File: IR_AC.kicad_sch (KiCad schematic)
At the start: 1 part

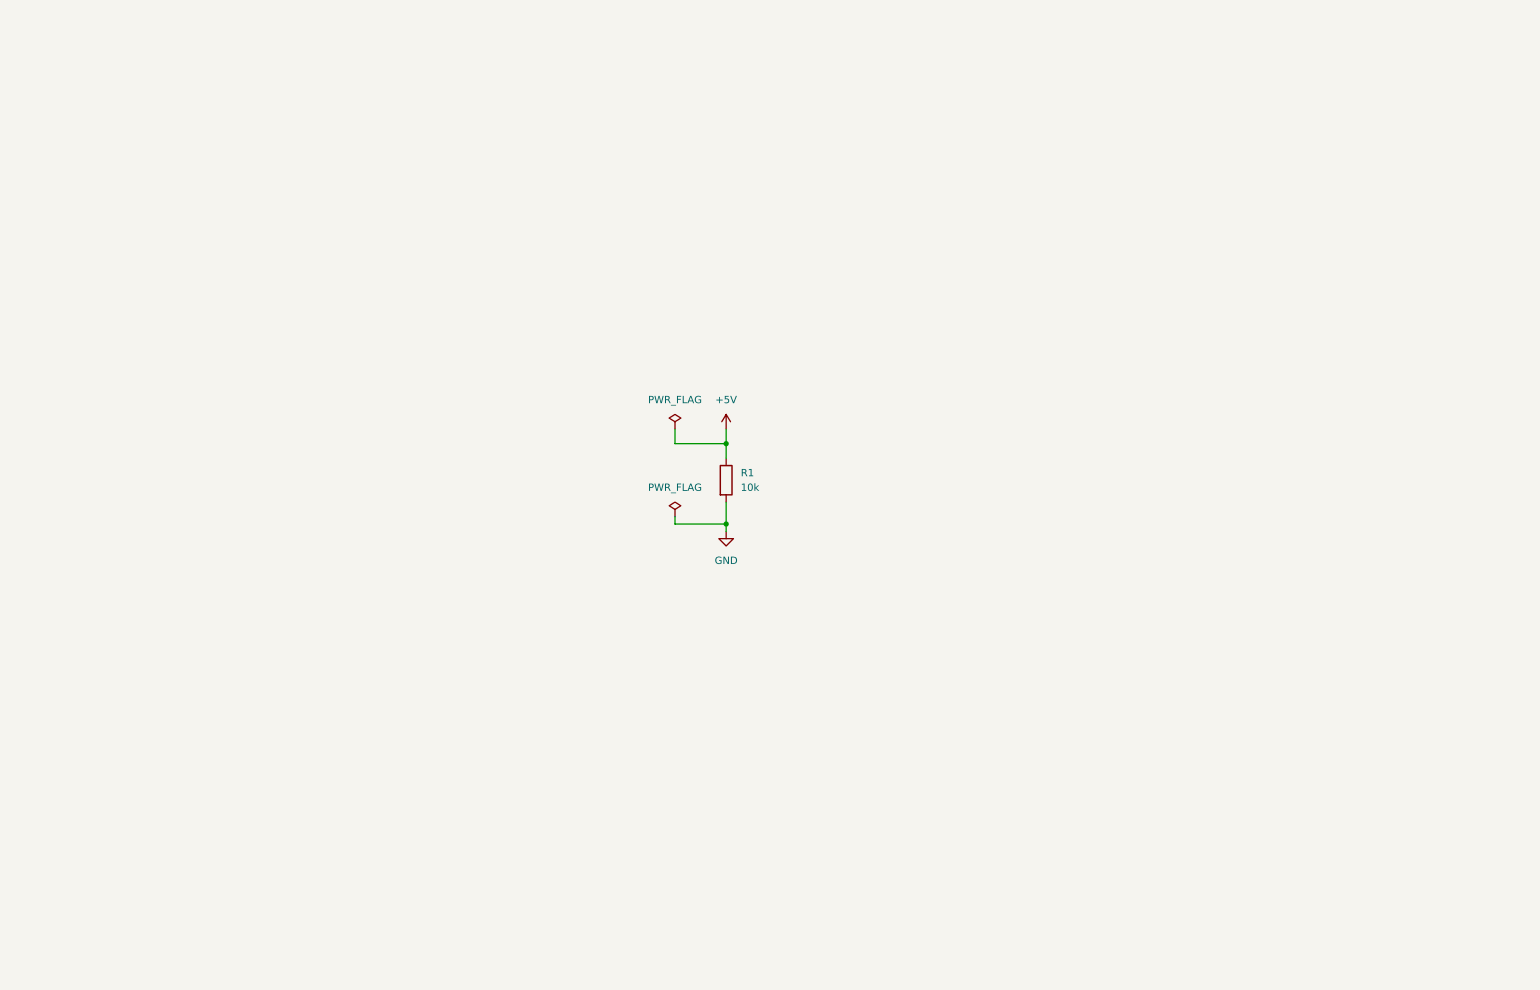
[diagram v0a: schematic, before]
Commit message: late night work on led current
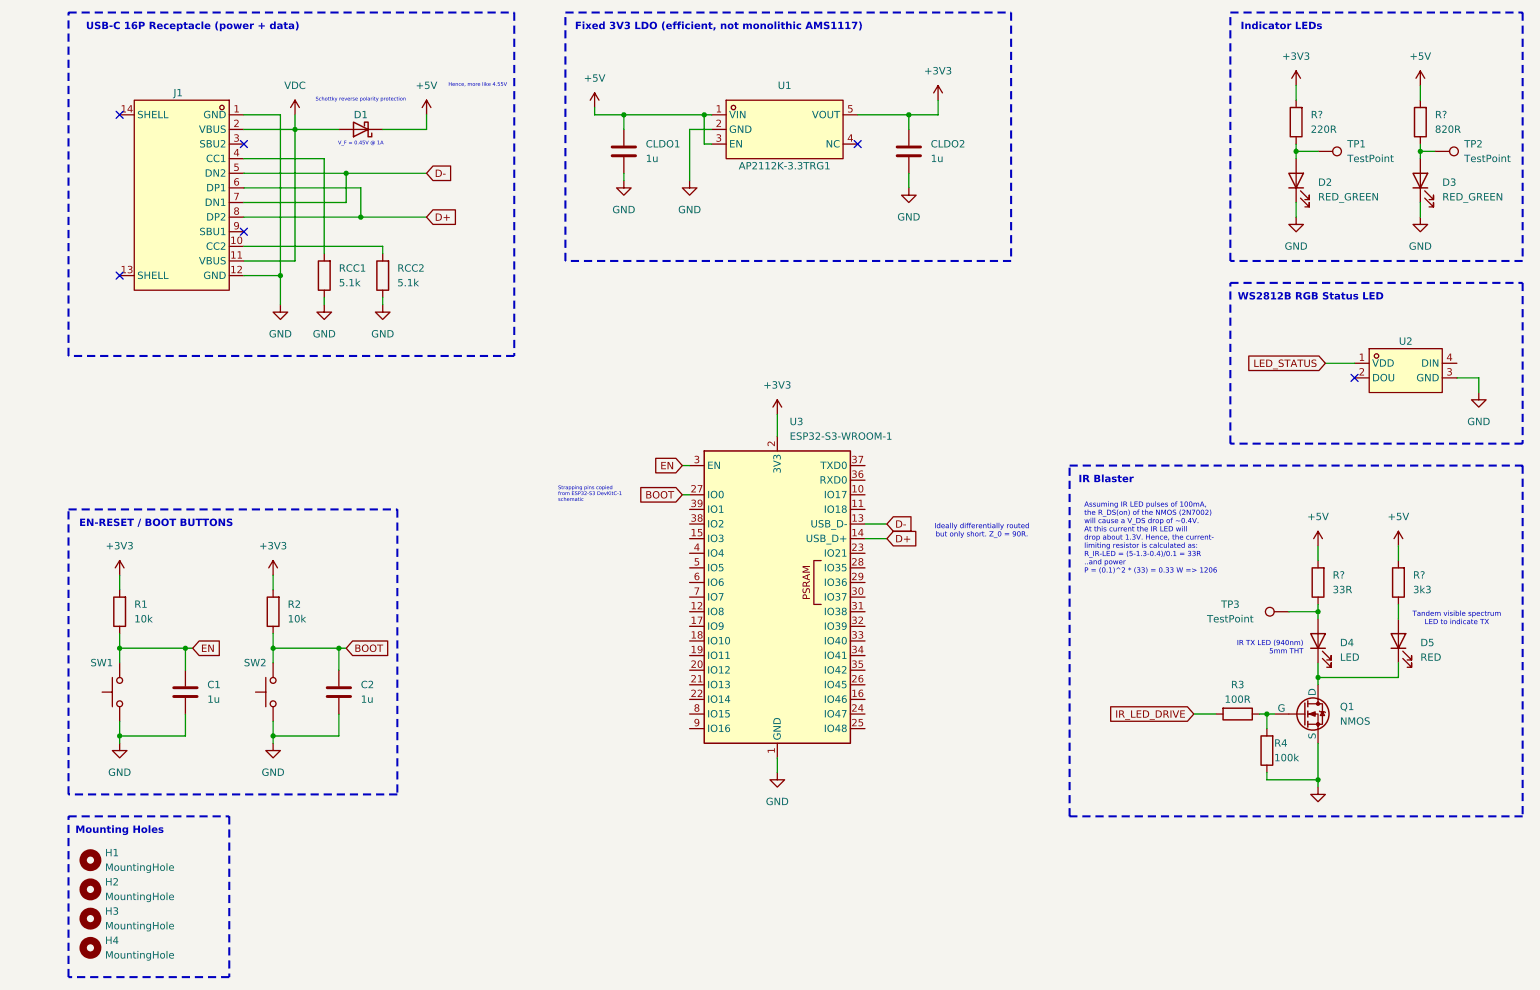
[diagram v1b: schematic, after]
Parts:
- added C1, C2: 1u, Capacitor_SMD:C_0603_1608Metric, symbol Device:C
- added CLDO1, CLDO2: 1u, Capacitor_SMD:C_0805_2012Metric, symbol Device:C
- added D1: 1N5819HW, LC_libz_foot:1N5819HW, symbol Device:D_Schottky
- added D2, D3: RED_GREEN, LED_SMD:LED_0805_2012Metric, symbol Device:LED
- added D4: LED, LC_libz_foot:IR_LED_TH_5MM, symbol Device:LED
- added D5: RED, LED_SMD:LED_0805_2012Metric, symbol Device:LED
- added H1, H2, H3, H4: MountingHole, MountingHole:MountingHole_3.2mm_M3, symbol Mechanical:MountingHole
- added J1: TYPE-C 16PIN 2MD(073), LC_libz_foot:USB-C-SMD_TYPE-C-6PIN-2MD-073, symbol LC_libz_sym:TYPE-C16PIN2MD(073)
- added Q1: NMOS, Package_TO_SOT_SMD:SOT-23, symbol Simulation_SPICE:NMOS
- added R2: 10k, Resistor_SMD:R_0603_1608Metric, symbol Device:R
- added R3: 100R, Resistor_SMD:R_0603_1608Metric, symbol Device:R
- added R4: 100k, Resistor_SMD:R_0603_1608Metric, symbol Device:R
- added R?: 3k3, Resistor_SMD:R_0603_1608Metric, symbol Device:R
- added R?: 220R, Resistor_SMD:R_0603_1608Metric, symbol Device:R
- added R?: 820R, Resistor_SMD:R_0603_1608Metric, symbol Device:R
- added R?: 33R, Resistor_SMD:R_1206_3216Metric, symbol Device:R
- added RCC1, RCC2: 5.1k, Resistor_SMD:R_0603_1608Metric, symbol Device:R
- added SW1, SW2: SW_Push, LC_libz_foot:BTN_L45_W45, symbol Switch:SW_Push
- added TP1, TP2, TP3: TestPoint, TestPoint:TestPoint_THTPad_D1.5mm_Drill0.7mm, symbol Connector:TestPoint
- added U1: AP2112K-3.3TRG1, LC_libz_foot:AP2112K-3.3, symbol LC_libz_sym:AP2112K-3.3TRG1
- added U2: WS2812B_5050, LC_libz_foot:WS2812B_5050, symbol LC_libz_sym:WS2812B_5050
- added U3: ESP32-S3-WROOM-1, RF_Module:ESP32-S3-WROOM-1, symbol RF_Module:ESP32-S3-WROOM-1
- R1: LCSC C2930027 -> C25804
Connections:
- net +5V: now also CLDO1.1, D1.1 (K), R?.2, R?.2, R?.2, U1.1 (VIN), U1.3 (EN); no longer R1.1
- net GND: now also C1.2, C2.2, CLDO1.2, CLDO2.2, D2.1 (K), D3.1 (K), J1.1 (GND), J1.12 (GND), Q1.3 (S), R4.1, RCC1.1, RCC2.1, SW1.1, SW2.1, U1.2 (GND), U2.3 (GND), U3.1 (GND), U3.40 (GND), U3.41 (GND); no longer R1.2
- new net: D3.2 (A), R?.1, TP2.1
- new net: D5.2 (A), R?.1
- new net: D2.2 (A), R?.1, TP1.1
- new net: J1.10 (CC2), RCC2.2
- new net: J1.4 (CC1), RCC1.2
- new net: D4.1 (K), D5.1 (K), Q1.1 (D)
- new net: Q1.2 (G), R3.1, R4.2
- new net: D4.2 (A), R?.1, TP3.1
- new net +3V3: CLDO2.1, R1.2, R2.2, R?.2, U1.5 (VOUT), U3.2 (3V3)
- new net BOOT: C2.1, R2.1, SW2.2, U3.27 (IO0)
- new net D+: J1.6 (DP1), J1.8 (DP2), U3.14 (USB_D+)
- new net D-: J1.5 (DN2), J1.7 (DN1), U3.13 (USB_D-)
- new net EN: C1.1, R1.1, SW1.2, U3.3 (EN)
- new net IR_LED_DRIVE: R3.2
- new net LED_STATUS: U2.1 (VDD)
- new net VDC: D1.2 (A), J1.11 (VBUS), J1.2 (VBUS)
- no-connect marks 0 -> 6
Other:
- note added: "Assuming IR LED pulses of 100mA, the R_DS(on) of the NMOS (2N7002) will cause a V_DS drop of ~0.4V. At this current the IR LED will drop about 1.3V. Hence, the current- limiting resistor is calculated as: R_IR-LED = (5-1.3-0.4)/0.1 = 33R ..and power P = (0.1)^2 * (33) = 0.33 W => 1206"
- note added: "EN-RESET / BOOT BUTTONS"
- note added: "Fixed 3V3 LDO (efficient, not monolithic AMS1117)"
- note added: "Hence, more like 4.55V"
- note added: "IR Blaster"
- note added: "IR TX LED (940nm) 5mm THT"
- note added: "Ideally differentially routed but only short. Z_0 = 90R."
- note added: "Indicator LEDs"
- note added: "Mounting Holes"
- note added: "Schottky reverse polarity protection"
- note added: "Strapping pins copied from ESP32-S3 DevKitC-1 schematic"
- note added: "Tandem visible spectrum LED to indicate TX"
- note added: "USB-C 16P Receptacle (power + data)"
- note added: "V_F = 0.45V @ 1A"
- note added: "WS2812B RGB Status LED"

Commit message: Finished schematic
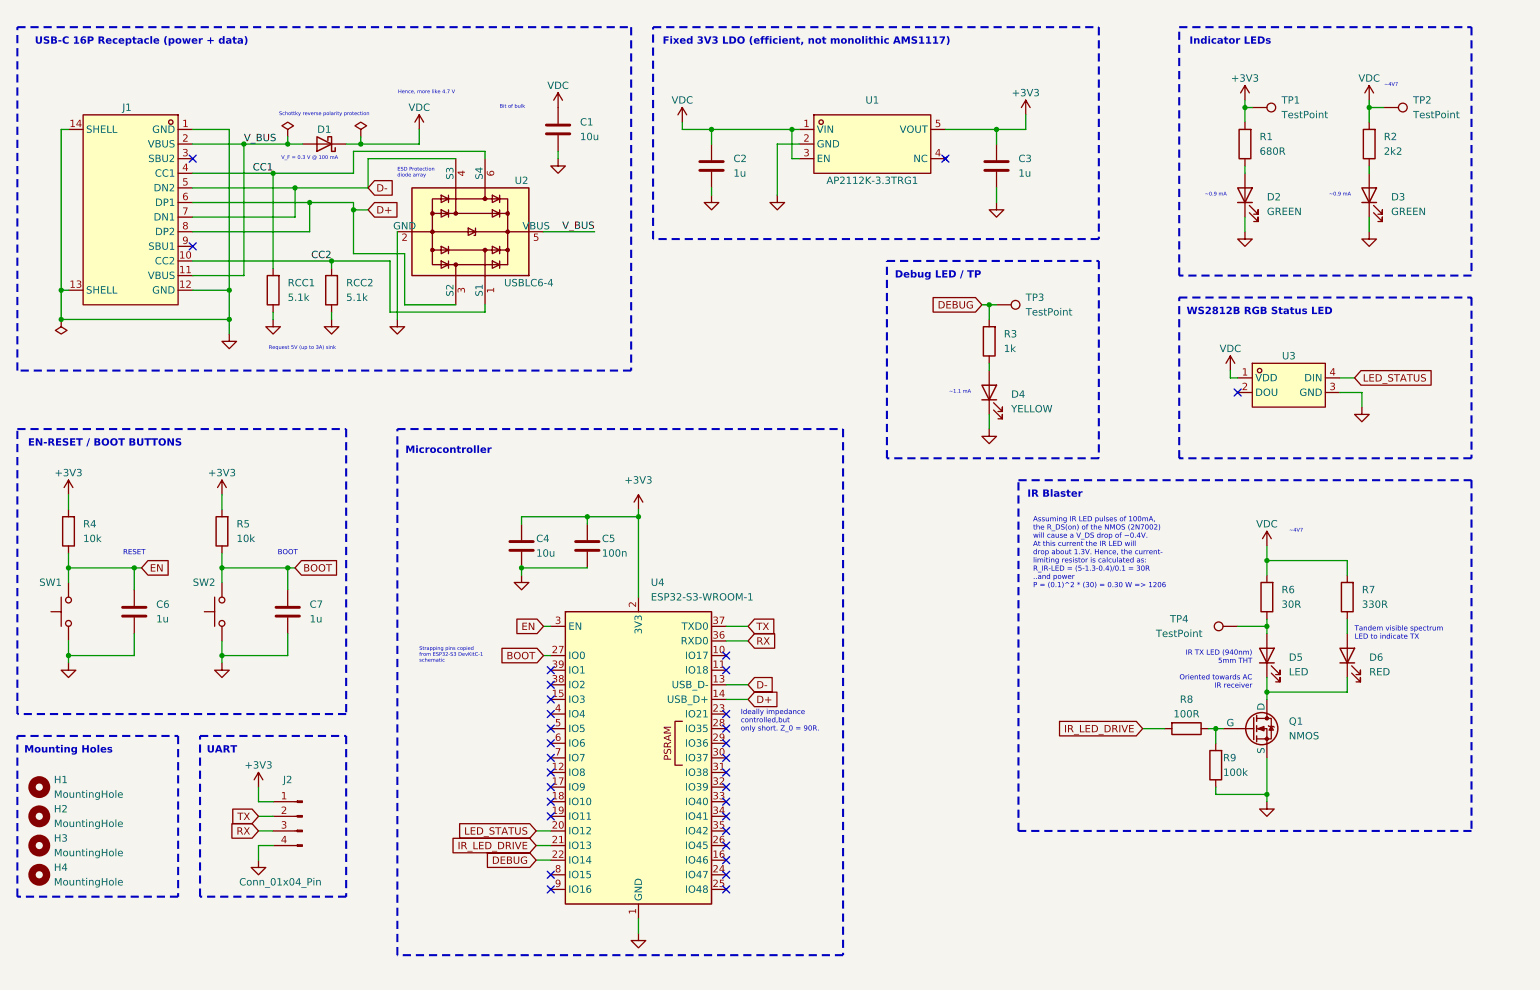
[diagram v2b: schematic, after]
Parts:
- added C1, C4: 10u, Capacitor_SMD:C_0805_2012Metric, symbol Device:C
- added C5: 100n, Capacitor_SMD:C_0402_1005Metric, symbol Device:C
- added D4: YELLOW, LED_SMD:LED_0805_2012Metric, symbol Device:LED
- added J2: Conn_01x04_Pin, libs:HDR-TH_4P-P2.54-V-M, symbol Connector:Conn_01x04_Pin
- added R3: 1k, Resistor_SMD:R_0603_1608Metric, symbol Device:R
- added TP3: TestPoint, TestPoint:TestPoint_THTPad_D1.5mm_Drill0.7mm, symbol Connector:TestPoint
- added U2: USBLC6-4, Package_TO_SOT_SMD:SOT-23-6, symbol Power_Protection:SRV05-4
- D2, D3: value RED_GREEN -> GREEN
- D6: renamed from D5; LCSC NULL -> C84256
- H1, H2, H3, H4: footprint MountingHole:MountingHole_3.2mm_M3 -> MountingHole:MountingHole_2.2mm_M2
- J1: footprint LC_libz_foot:USB-C-SMD_TYPE-C-6PIN-2MD-073 -> libs:USB-C-SMD_TYPE-C-6PIN-2MD-073
- R1: renamed from R?; value 220R -> 680R; LCSC C22962 -> C23228
- R2: renamed from R?; value 820R -> 2k2; LCSC C23253 -> C4190
- R6: renamed from R?; value 33R -> 30R; LCSC C18005 -> C25373
- R7: renamed from R?; value 3k3 -> 330R; LCSC C22978 -> C23138
- SW1, SW2: footprint LC_libz_foot:BTN_L45_W45 -> (none); LCSC C455243 -> C720477
- U1: footprint LC_libz_foot:AP2112K-3.3 -> libs:SOT-25-5_L2.9-W1.6-P0.95-LS2.8-BL
- renumbered CLDO1 to C2, CLDO2 to C3, C1 to C6, C2 to C7, D4 to D5, R1 to R4, R2 to R5, R3 to R8, R4 to R9, TP3 to TP4, U2 to U3, U3 to U4
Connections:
- net +5V is gone; now on net VDC: C2.1, D1.1 (K), R2.2, R6.2, R7.2, U1.1 (VIN), U1.3 (EN)
- net +3V3: now also TP1.1, C4.1, C5.1, J2.1 (Pin_1)
- net D+: now also U2.3 (S2)
- net D-: now also U2.4 (S3)
- net GND: now also J1.13 (SHELL), J1.14 (SHELL), C1.2, C4.2, C5.2, D4.1 (K), J2.4 (Pin_4), U2.2 (GND)
- net IR_LED_DRIVE: now also U4.21 (IO13)
- net LED_STATUS: now also U3.4 (DIN), U4.20 (IO12); no longer U3.1 (VDD)
- net VDC: now also TP2.1, U3.1 (VDD), C1.1; no longer D1.2 (A), J1.11 (VBUS), J1.2 (VBUS)
- net at D3.2 (A), R2.1: no longer TP2.1
- net at D2.2 (A), R1.1: no longer TP1.1
- net CC2: now reaches J1.10 (CC2), RCC2.2
- net CC2: now also U2.1 (S1)
- net CC1: now reaches J1.4 (CC1), RCC1.2
- net CC1: now also U2.6 (S4)
- net DEBUG: now reaches U4.22 (IO14)
- net DEBUG: now also R3.2, TP3.1
- net RX: now reaches U4.36 (RXD0)
- net RX: now also J2.3 (Pin_3)
- net TX: now reaches U4.37 (TXD0)
- net TX: now also J2.2 (Pin_2)
- new net: D4.2 (A), R3.1
- new net V_BUS: D1.2 (A), J1.11 (VBUS), J1.2 (VBUS), U2.5 (VBUS)
- no-connect marks 6 -> 32
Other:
- note added: "Assuming IR LED pulses of 100mA, the R_DS(on) of the NMOS (2N7002) will cause a V_DS drop of ~0.4V. At this current the IR LED will drop about 1.3V. Hence, the current- limiting resistor is calculated as: R_IR-LED = (5-1.3-0.4)/0.1 = 30R ..and power P = (0.1)^2 * (30) = 0.30 W => 1206"
- note added: "BOOT"
- note added: "Bit of bulk"
- note added: "Debug LED / TP"
- note added: "ESD Protection diode array"
- note added: "Hence, more like 4.7 V"
- note added: "IR TX LED (940nm) 5mm THT Oriented towards AC IR receiver"
- note added: "Ideally impedance controlled,but only short. Z_0 = 90R."
- note added: "Microcontroller"
- note added: "RESET"
- note added: "Request 5V (up to 3A) sink"
- note added: "UART"
- note added: "V_F = 0.3 V @ 100 mA"
- note added: "~0.9 mA"
- note added: "~1.1 mA"
- note added: "~4V7"
- note removed: "Assuming IR LED pulses of 100mA, the R_DS(on) of the NMOS (2N7002) will cause a V_DS drop of ~0.4V. At this current the IR LED will drop about 1.3V. Hence, the current- limiting resistor is calculated as: R_IR-LED = (5-1.3-0.4)/0.1 = 33R ..and power P = (0.1)^2 * (33) = 0.33 W => 1206"
- note removed: "Hence, more like 4.55V"
- note removed: "IR TX LED (940nm) 5mm THT"
- note removed: "Ideally differentially routed but only short. Z_0 = 90R."
- note removed: "V_F = 0.45V @ 1A"
- moved on the sheet: C2, C3, C6, C7, D1, D2, D3, D5, D6, H1, J1, Q1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
